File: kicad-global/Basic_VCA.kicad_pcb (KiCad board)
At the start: 2 copper layers, 172.5 x 128.5 mm, 151 parts, among them J1 CV, J10 In, J11 Out, J12 Conn_Circuit, J13 Conn_Jack, J14 CV, J15 In, J16 Out, J17 Conn_Circuit, J18 Conn_Jack, J19 CV, J2 In, J20 In, J21 Out, J22 Conn_Circuit, J23 Conn_Jack, J3 Conn_Circuit, J4 Conn_power, J5 Conn_Jack, J6 Conn_power, J7 Out, J8 Power Input, J9 CV, Q1 2N3904, Q2 2N3906, Q3 2N3904, Q4 2N3906, Q5 2N3904, Q6 2N3906, Q7 2N3904, Q8 2N3906, SW1 log/lin, SW2 log/lin, SW3 log/lin, SW4 log/lin, U1 TL074, U2 LM13700, U3 LM13700, U4 TL074

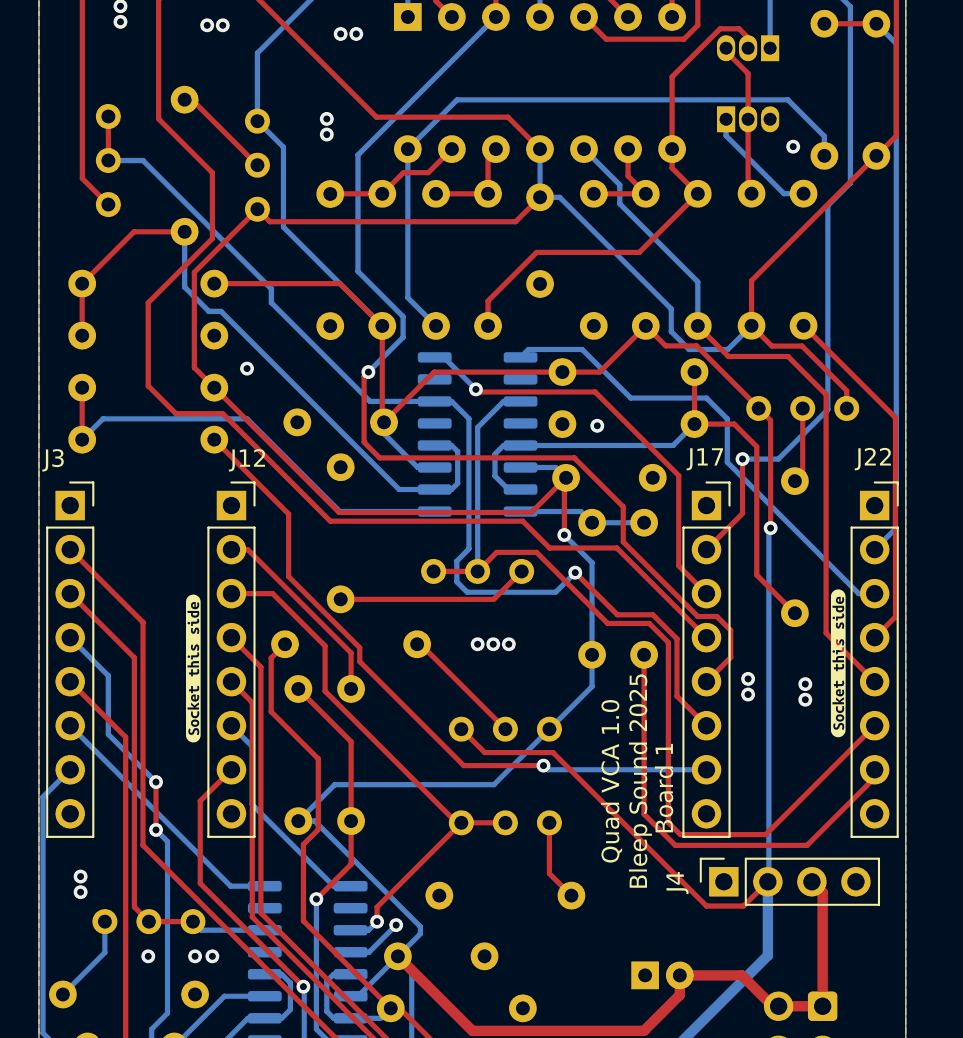
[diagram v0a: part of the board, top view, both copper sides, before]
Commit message: updated doc
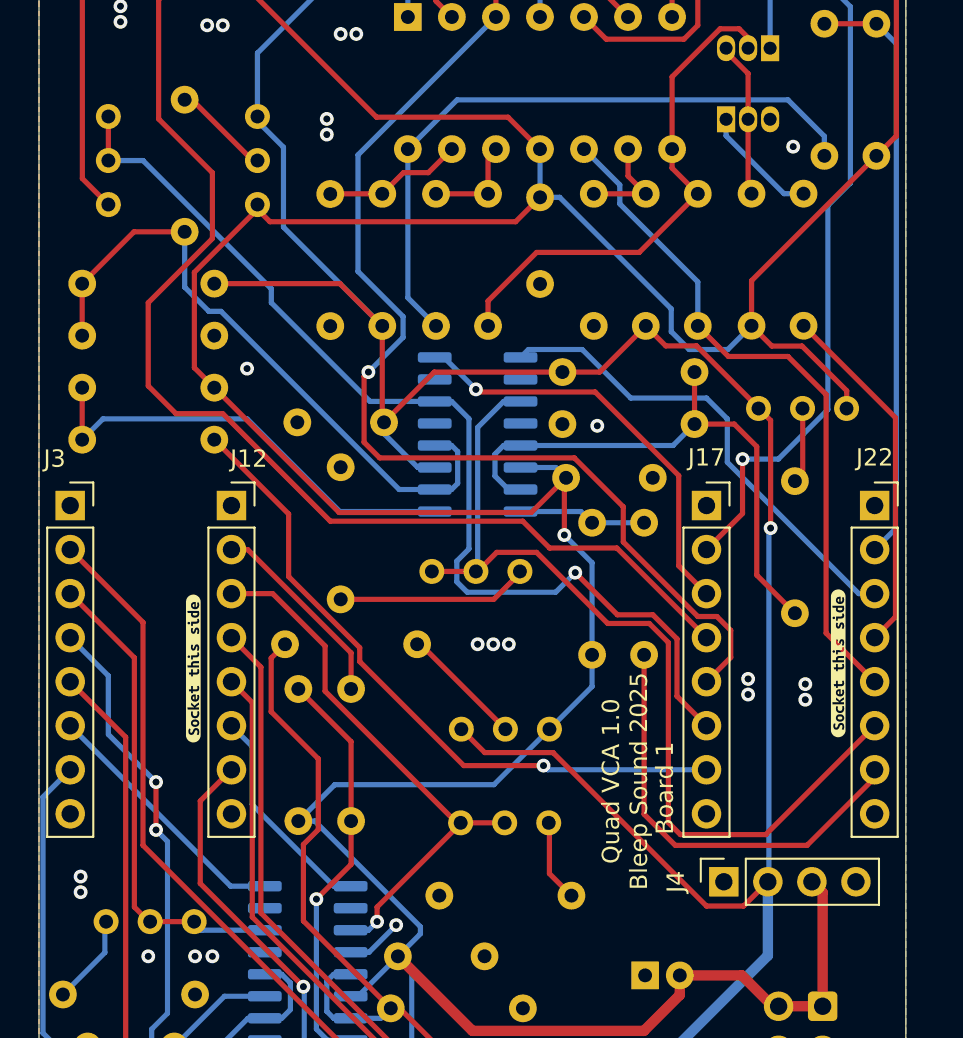
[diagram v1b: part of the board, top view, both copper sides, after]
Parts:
- Bias_adjust1, Bias_adjust2, Bias_adjust3, Bias_adjust4, Trim1, Trim2, Trim3, Trim4: footprint Potentiometer_THT:Potentiometer_Bourns_3386C_Horizontal -> Potentiometer_THT:Potentiometer_Bourns_3296W_Vertical
- moved Bias_adjust3 0.27 mm to (67.1, 54.3), turned to 90 degrees
- moved Trim4 0.10 mm to (77.2, 80.5), turned to 180 degrees
- moved Trim1 0.07 mm to (63.5, 100.7), turned to 0 degrees
- turned Trim2 to 180 degrees
- turned Bias_adjust4 to 180 degrees
- turned Bias_adjust1 to 0 degrees
- turned Bias_adjust2 to 180 degrees
- turned Trim3 to 90 degrees
